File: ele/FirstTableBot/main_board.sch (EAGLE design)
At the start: 118 parts, among them IC1 MCP602ST, X4 POWER_IN

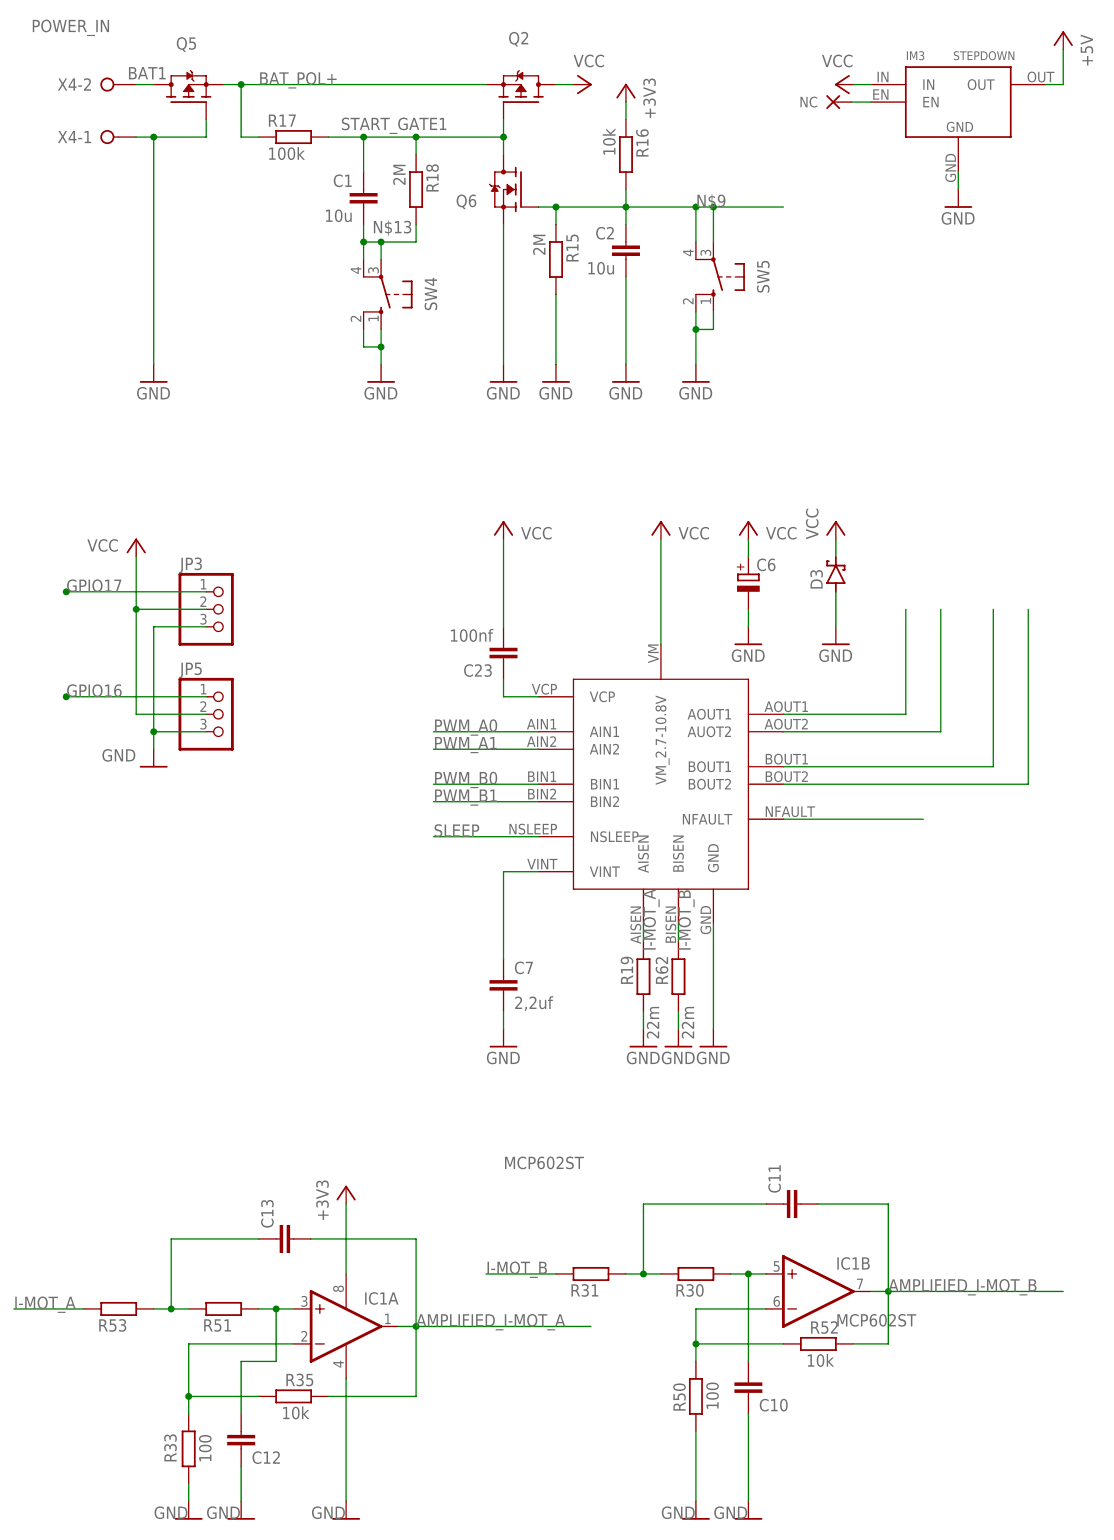
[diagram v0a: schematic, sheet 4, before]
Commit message: napájení z powerbanki
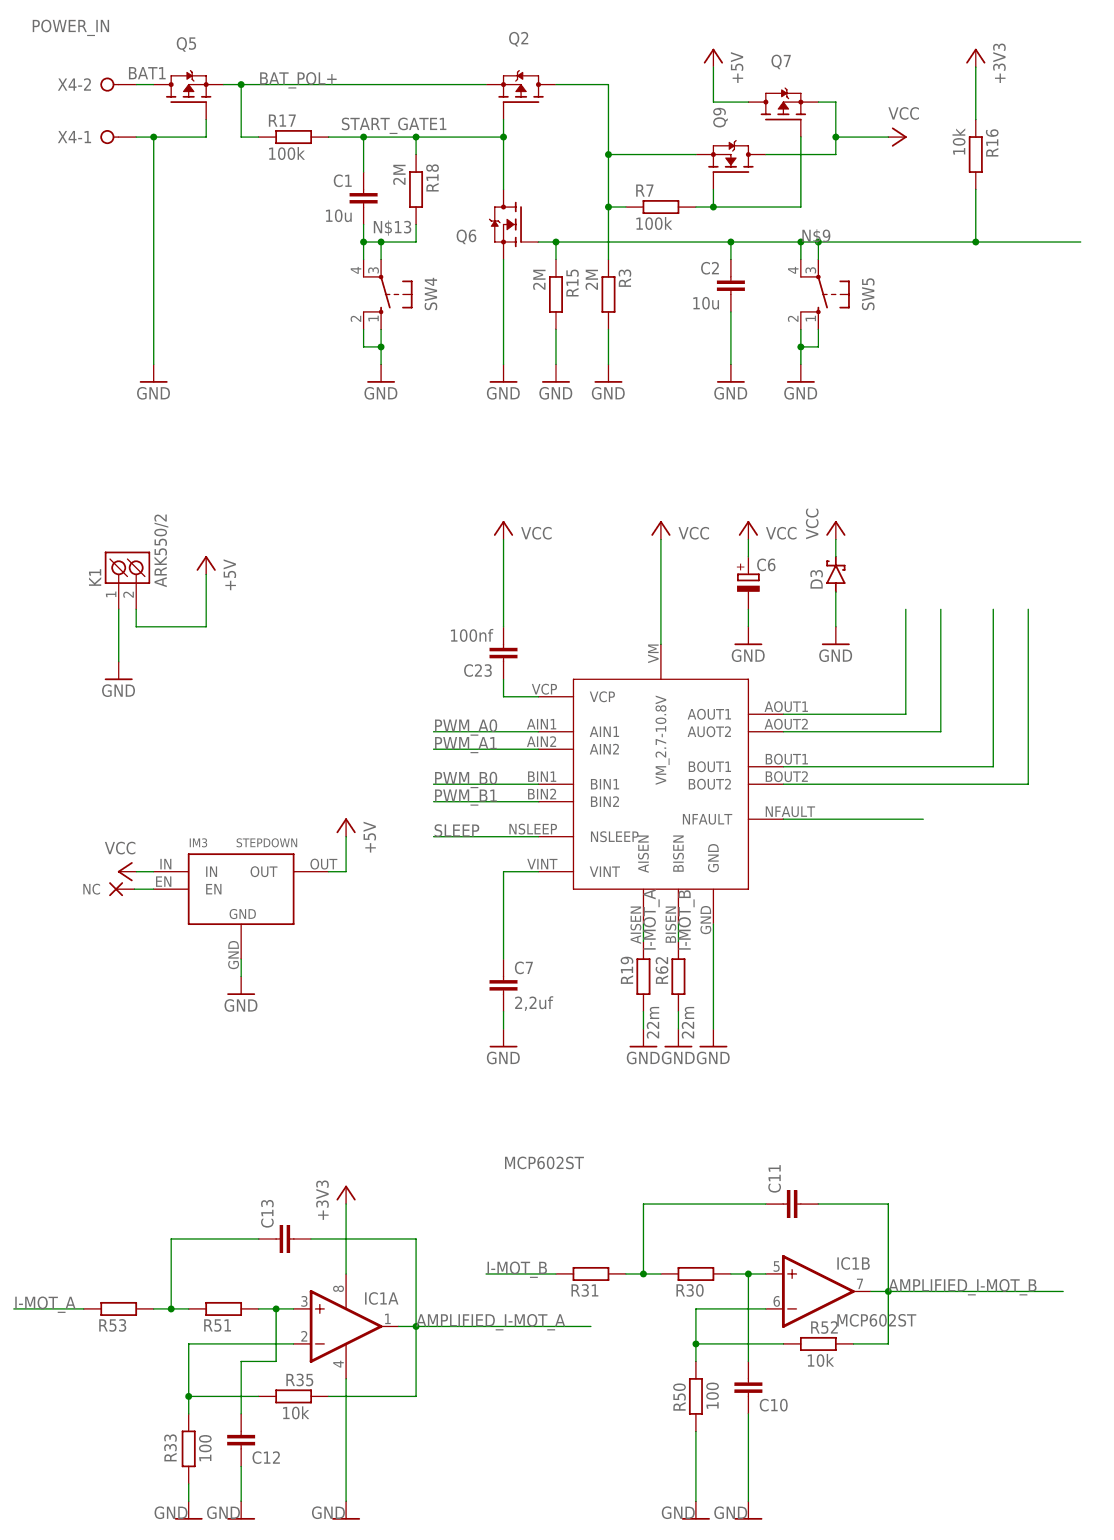
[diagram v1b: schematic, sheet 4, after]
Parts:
- added K1: ARK550/2, #PaJa_konektory:ARK550/2
- added Q7: (no value), transistors:P-MOSFET-MLP_HS
- added Q9: (no value), transistors:N-MOSFET-SOT23-GSD
- added R3: 2M, rcl_upravena:R-EU_R0805
- added R7: 100k, rcl_upravena:R-EU_R0805
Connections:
- new net N$35: Q7.G, Q9.G, R7.2
- new net N$7: Q2.D, Q9.S, R3.1, R7.1
- net +5V: now also JP3.2, JP5.2, K1.K2, Q7.D
- net GND: now also K1.K1, R3.2
- net VCC: now also Q7.S, Q9.D; no longer JP3.2, JP5.2, Q2.D
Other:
- moved on the sheet: C2, IM3, Q6, R15, R16, SW5

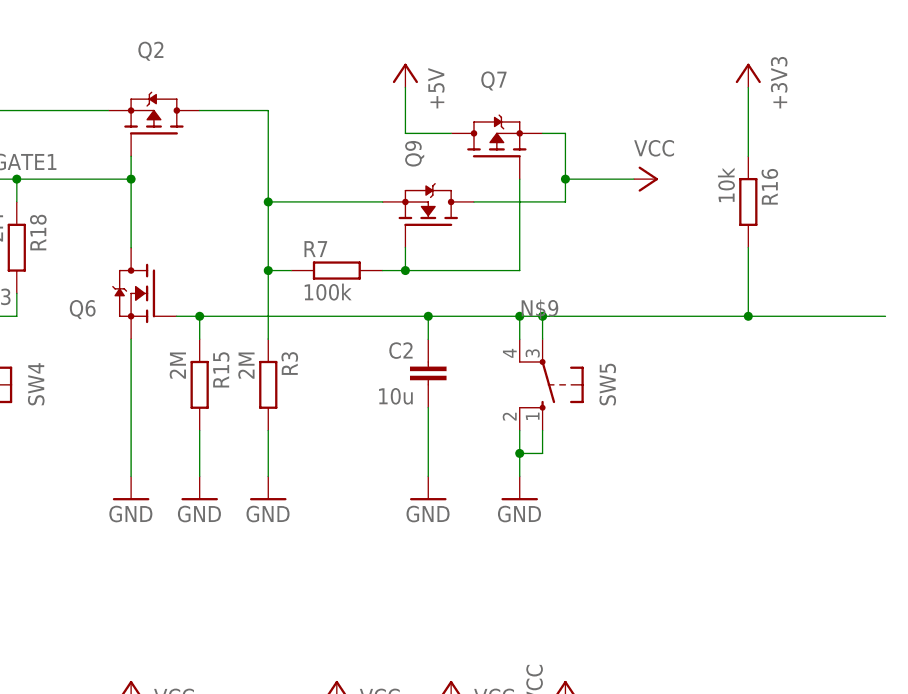
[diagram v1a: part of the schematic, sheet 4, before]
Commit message: nastrel_textu
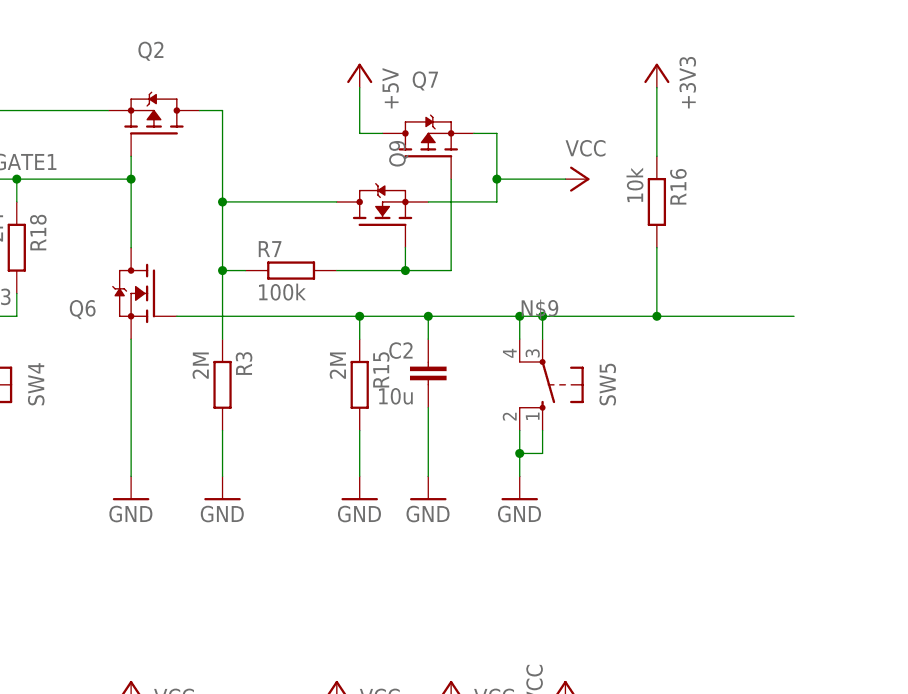
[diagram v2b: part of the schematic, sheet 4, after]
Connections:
- net N$7: now also Q9.D; no longer Q9.S
- net VCC: now also Q9.S; no longer Q9.D
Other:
- moved on the sheet: Q7, Q9, R15, R16, R3, R7
